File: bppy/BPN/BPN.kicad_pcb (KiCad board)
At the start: 2 copper layers, 61.6 x 68.2 mm, 33 parts, among them J1 USB_C_Receptacle_PowerOnly_6P, J2 Valve, J3 Pumpe, Q1 2N2219, Q2 IRLIZ44N, U1 LM317_TO-220, U2 NCP1117-3.3_SOT223, U3 Pico, U4 NJM4560, U5 AMS6915

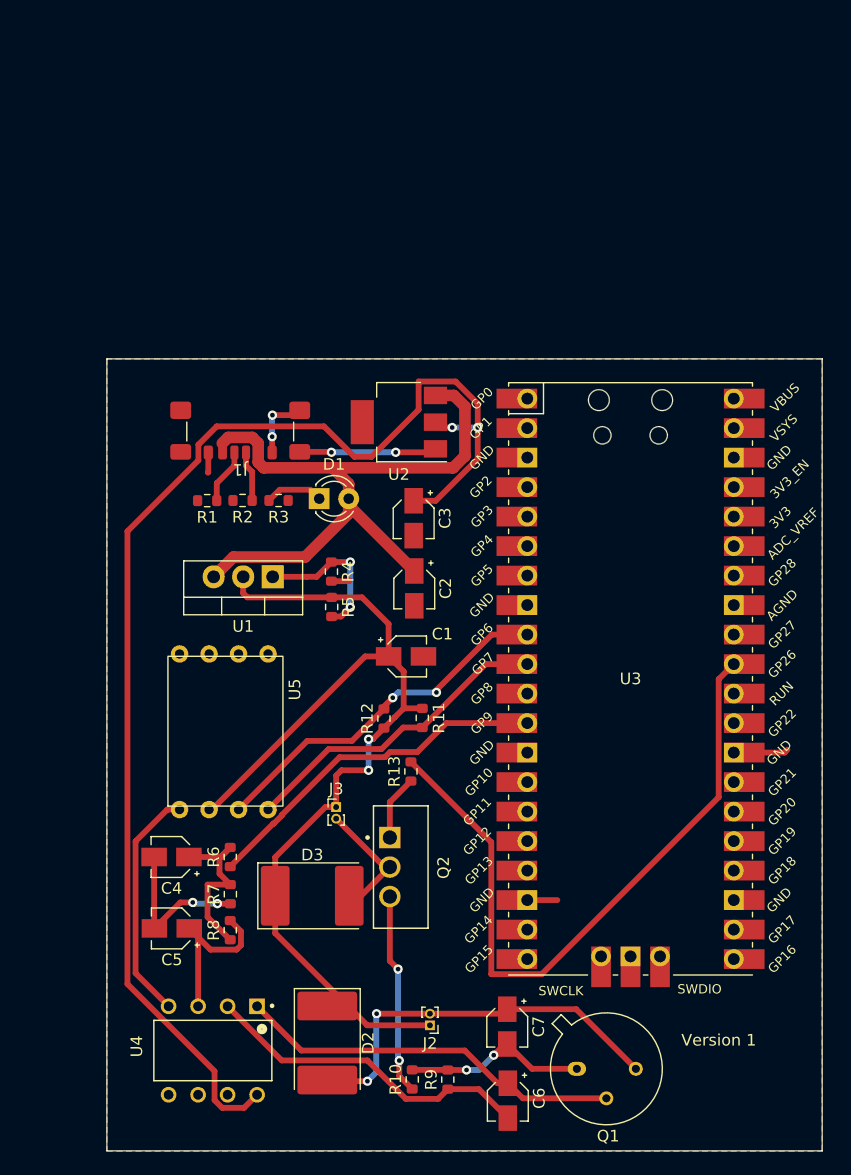
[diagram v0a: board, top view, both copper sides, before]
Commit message: with simulator
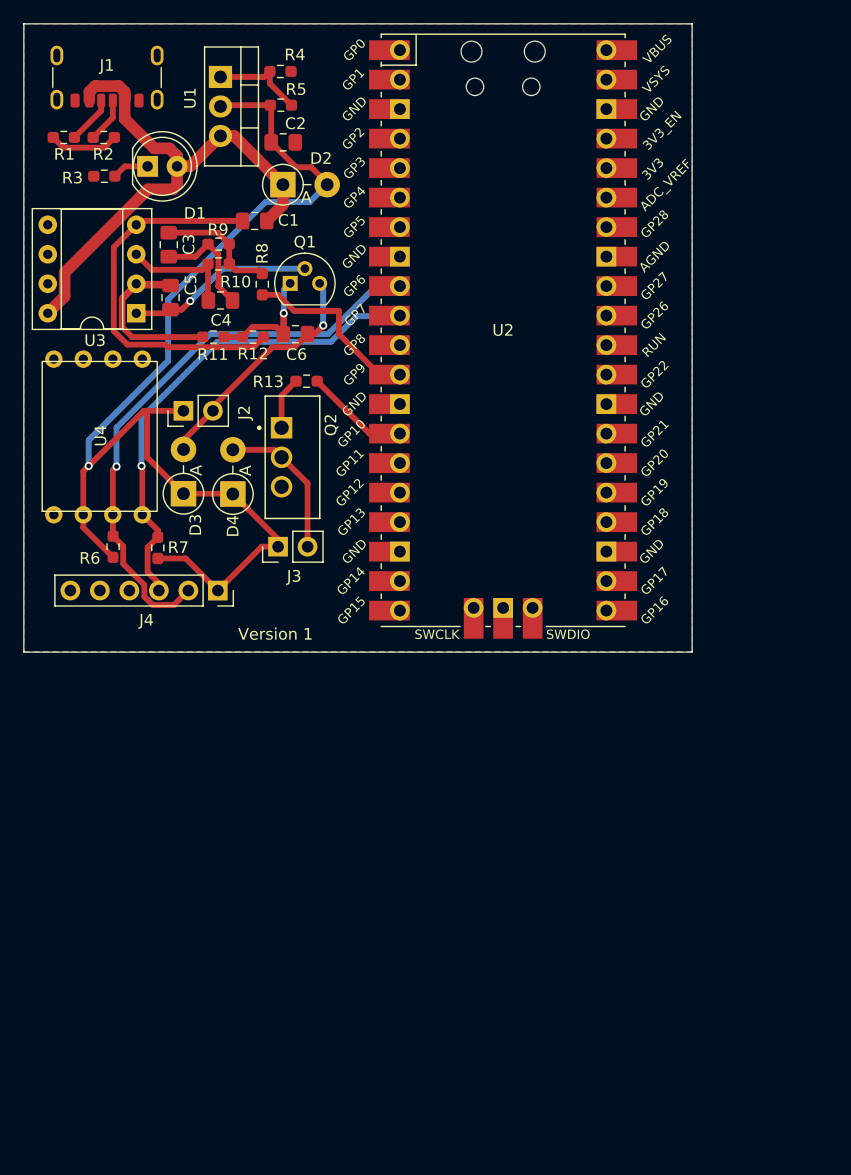
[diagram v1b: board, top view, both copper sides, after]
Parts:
- removed C7: 100n, Capacitor_SMD:CP_Elec_3x5.3
- removed U5: AMS6915, MedVet_FP:AMS_6915_FP
- added D4: 1N4002, Diode_THT:D_DO-41_SOD81_P3.81mm_Vertical_AnodeUp, F.Cu at (157.8, 86.4)
- added J4: Sensor_2, Connector_PinSocket_2.54mm:PinSocket_1x06_P2.54mm_Vertical, F.Cu at (156.6, 94.8)
- C1: value C_Polarized -> 0.1u; footprint Capacitor_SMD:CP_Elec_3x5.3 -> Capacitor_SMD:C_0805_2012Metric_Pad1.18x1.45mm_HandSolder
- C2, C3: value 10u -> 1u; footprint Capacitor_SMD:CP_Elec_3x5.3 -> Capacitor_SMD:C_0805_2012Metric_Pad1.18x1.45mm_HandSolder
- C4: value 1u -> 100n; footprint Capacitor_SMD:CP_Elec_3x5.3 -> Capacitor_SMD:C_0805_2012Metric_Pad1.18x1.45mm_HandSolder
- C5: footprint Capacitor_SMD:CP_Elec_3x5.3 -> Capacitor_SMD:C_0805_2012Metric_Pad1.18x1.45mm_HandSolder
- C6: value 100n -> 0.1u; footprint Capacitor_SMD:CP_Elec_3x5.3 -> Capacitor_SMD:C_0805_2012Metric_Pad1.18x1.45mm_HandSolder
- D1: footprint LED_THT:LED_D3.0mm_FlatTop -> LED_THT:LED_D5.0mm
- D2, D3: value 1N4001 -> 1N4002; footprint Diode_SMD:D_3220_8050Metric -> Diode_THT:D_DO-41_SOD81_P3.81mm_Vertical_AnodeUp
- J1: footprint Connector_USB:USB_C_Receptacle_GCT_USB4135-GF-A_6P_TopMnt_Horizontal -> Connector_USB:USB_C_Receptacle_GCT_USB4125-xx-x-0190_6P_TopMnt_Horizontal
- J2, J3: footprint Connector_PinHeader_1.00mm:PinHeader_1x02_P1.00mm_Vertical -> Connector_PinHeader_2.54mm:PinHeader_1x02_P2.54mm_Vertical
- Q1: value 2N2219 -> 2N2222A; footprint Package_TO_SOT_THT:TO-39-3 -> Package_TO_SOT_THT:TO-92
- R1, R2, R8: footprint Resistor_SMD:R_0603_1608Metric -> Resistor_SMD:R_0603_1608Metric_Pad0.98x0.95mm_HandSolder
- R10: value 10 -> 100k; footprint Resistor_SMD:R_0603_1608Metric -> Resistor_SMD:R_0603_1608Metric_Pad0.98x0.95mm_HandSolder
- R11: value 4.7k -> 100k; footprint Resistor_SMD:R_0603_1608Metric -> Resistor_SMD:R_0603_1608Metric_Pad0.98x0.95mm_HandSolder
- R12: value 4.7k -> 10; footprint Resistor_SMD:R_0603_1608Metric -> Resistor_SMD:R_0603_1608Metric_Pad0.98x0.95mm_HandSolder
- R13: value 1.2k -> 1k; footprint Resistor_SMD:R_0603_1608Metric -> Resistor_SMD:R_0603_1608Metric_Pad0.98x0.95mm_HandSolder
- R3: value 2.5k -> 2.52k; footprint Resistor_SMD:R_0603_1608Metric -> Resistor_SMD:R_0603_1608Metric_Pad0.98x0.95mm_HandSolder
- R4: value 820 -> 390; footprint Resistor_SMD:R_0603_1608Metric -> Resistor_SMD:R_0603_1608Metric_Pad0.98x0.95mm_HandSolder
- R5: value 510 -> 240; footprint Resistor_SMD:R_0603_1608Metric -> Resistor_SMD:R_0603_1608Metric_Pad0.98x0.95mm_HandSolder
- R6: value 100k -> 4.7k; footprint Resistor_SMD:R_0603_1608Metric -> Resistor_SMD:R_0603_1608Metric_Pad0.98x0.95mm_HandSolder
- R7: value 33k -> 4.7k; footprint Resistor_SMD:R_0603_1608Metric -> Resistor_SMD:R_0603_1608Metric_Pad0.98x0.95mm_HandSolder
- R9: value 100k -> 33k; footprint Resistor_SMD:R_0603_1608Metric -> Resistor_SMD:R_0603_1608Metric_Pad0.98x0.95mm_HandSolder
- U1: value LM317_TO-220 -> LM317
- U2: value NCP1117-3.3_SOT223 -> Pico; footprint Package_TO_SOT_SMD:SOT-223 -> MCU_RaspberryPi_and_Boards:RPi_Pico_SMD_TH
- U3: value Pico -> NJM2904D; footprint MCU_RaspberryPi_and_Boards:RPi_Pico_SMD_TH -> Package_DIP:DIP-8_W7.62mm_Socket
- U4: value NJM4560 -> AMS6915; footprint NJM4560D:DIP762W46P254L880H425Q8 -> MedVet_FP:AMS_6915_FP
- moved R9 74.6 mm to (156.6, 64.9), turned to 0 degrees
- moved D2 74.0 mm to (162.2, 59.8), turned to 0 degrees
- moved R10 72.2 mm to (156.6, 66.6), turned to 180 degrees
- moved Q1 72.0 mm to (162.8, 68.3)
- moved C6 68.5 mm to (163.2, 72.7), turned to 180 degrees
- moved J2 57.0 mm to (153.6, 79.3), turned to 90 degrees
- moved R8 55.7 mm to (160.4, 68.4)
- moved C5 54.3 mm to (152.5, 69.5), turned to 90 degrees
- moved U3 52.9 mm to (149.5, 70.9), turned to 180 degrees
- moved U4 51.9 mm to (144.3, 83.8), turned to 90 degrees
- moved C4 48.1 mm to (156.8, 69.8), turned to 0 degrees
- moved R5 43.4 mm to (162.0, 53.0), turned to 0 degrees
- moved R4 43.3 mm to (161.9, 50.1), turned to 0 degrees
- moved U1 43.3 mm to (156.8, 50.5), turned to -90 degrees
- moved C2 40.0 mm to (162.2, 56.2), turned to 0 degrees
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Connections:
- C1 pad 1: +3V3 -> +5V
- C2 pad 1: +5V -> +3.3V
- C3 pad 1: VDD -> Net-(C3-Pad1)
- C3 pad 2: GND -> Net-(C3-Pad2)
- C4 pad 1: Net-(C4-Pad1) -> Net-(U3A-+)
- C4 pad 2: Net-(C4-Pad2) -> Net-(C3-Pad2)
- C5 pad 1: Net-(U4A-+) -> Net-(Q1-B)
- C5 pad 2: Net-(C4-Pad2) -> Net-(U3A--)
- C6 pad 1: Net-(Q1-B) -> Net-(D3-A)
- C6 pad 2: Net-(U4A--) -> Net-(Q1-E)
- D2 pad 1: +3V3 -> +5V
- D2 pad 2: Net-(D2-A) -> +3.3V
- D3 pad 1: +3V3 -> +3.3V
- J2 pad 1: +3V3 -> +3.3V
- J2 pad 2: Net-(D2-A) -> Net-(D3-A)
- J3 pad 1: +3V3 -> +3.3V
- J3 pad 2: Net-(D3-A) -> Net-(D4-A)
- Q1 pad 3: Net-(D2-A) -> Net-(D3-A)
- Q2 pad 2: Net-(D3-A) -> Net-(D4-A)
- R10 pad 1: GND -> Net-(C3-Pad1)
- R10 pad 2: Net-(Q1-E) -> Net-(U3A-+)
- R11 pad 1: +3V3 -> Net-(U3A--)
- R11 pad 2: /SCL -> Net-(Q1-E)
- R12 pad 1: +3V3 -> GND
- R12 pad 2: /SDA -> Net-(Q1-E)
- R5 pad 1: +3V3 -> +3.3V
- R6 pad 1: /Valve -> +3.3V
- R6 pad 2: Net-(C4-Pad1) -> /SDA
- R7 pad 1: Net-(C4-Pad2) -> +3.3V
- R7 pad 2: Net-(C4-Pad1) -> /SCL
- R8 pad 1: Net-(C4-Pad1) -> /Valve
- R8 pad 2: Net-(U4A-+) -> Net-(C3-Pad1)
- R9 pad 1: Net-(U4A--) -> Net-(C3-Pad2)
- R9 pad 2: Net-(Q1-E) -> Net-(C3-Pad1)
- U1 pad 2: +3V3 -> +3.3V
- U2 pad 1: GND -> unconnected-(U2-GPIO0-Pad1)
- U2 pad 2: VDD -> unconnected-(U2-GPIO1-Pad2)
- U2 pad 3: +5V -> GND
- U2 pad 4: (no net) -> unconnected-(U2-GPIO2-Pad4)
- U3 pad 1: unconnected-(U3-GPIO0-Pad1) -> Net-(Q1-B)
- U3 pad 2: unconnected-(U3-GPIO1-Pad2) -> Net-(U3A--)
- U3 pad 3: GND -> Net-(U3A-+)
- U3 pad 4: unconnected-(U3-GPIO2-Pad4) -> GND
- U3 pad 5: unconnected-(U3-GPIO3-Pad5) -> (no net)
- U3 pad 6: unconnected-(U3-GPIO4-Pad6) -> (no net)
- U3 pad 7: unconnected-(U3-GPIO5-Pad7) -> (no net)
- U3 pad 8: GND -> +5V
- U4 pad 1: Net-(Q1-B) -> GND
- U4 pad 2: Net-(U4A--) -> +3.3V
- U4 pad 3: Net-(U4A-+) -> /SDA
- U4 pad 4: GND -> /SCL
- U4 pad 5: (no net) -> unconnected-(U4-NC-Pad5)
- U4 pad 6: (no net) -> unconnected-(U4-NC-Pad6)
- U4 pad 7: (no net) -> unconnected-(U4-NC-Pad7)
- U4 pad 8: VDD -> unconnected-(U4-NC-Pad8)
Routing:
- net VDD: track 112.8 -> 0.00 mm, vias 2 -> 0
- net +3.3V: track 0.00 -> 101.0 mm, vias 0 -> 1
- net +3V3: track 88.0 -> 0.00 mm, vias 2 -> 0
- net /Pump: track 59.0 -> 8.99 mm
- net Net-(D2-A): track 34.4 -> 0.00 mm, vias 2 -> 0
- net Net-(U4A--): track 28.9 -> 0.00 mm
- net GND: track 67.6 -> 39.1 mm, vias 6 -> 0
- net Net-(U3A--): track 0.00 -> 22.0 mm
- net /SDA: track 31.3 -> 50.2 mm, vias 2 -> 1
- net Net-(Q1-B): track 34.0 -> 16.9 mm, vias 0 -> 1
- net /SCL: track 27.5 -> 43.0 mm, vias 0 -> 1
- net Net-(C4-Pad1): track 15.4 -> 0.00 mm
- net Net-(U4A-+): track 14.9 -> 0.00 mm
- net /Valve: track 30.7 -> 15.9 mm
- net Net-(C4-Pad2): track 13.7 -> 0.00 mm, vias 2 -> 0
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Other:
- board size 61.6 x 68.2 mm -> 57.6 x 54.1 mm
